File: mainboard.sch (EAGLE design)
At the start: 75 parts, among them Q3 MOSFET-PCHANNEL, Q4 MOSFET-PCHANNEL, T1 SINGLE_NCHAN_FET, T2 MOSFET_PCHAN_20A, T3 SINGLE_NCHAN_FET, T4 MOSFET_PCHAN_20A, T5 SINGLE_NCHAN_FET, T6 MOSFET_PCHAN_20A, U1 LT3688, U2 TEENSY_3.0+4, U3 RFM23BP, U4 HMC5883LSMD, U5 ITG-3200, U9 MIC803-31D3VM3TR

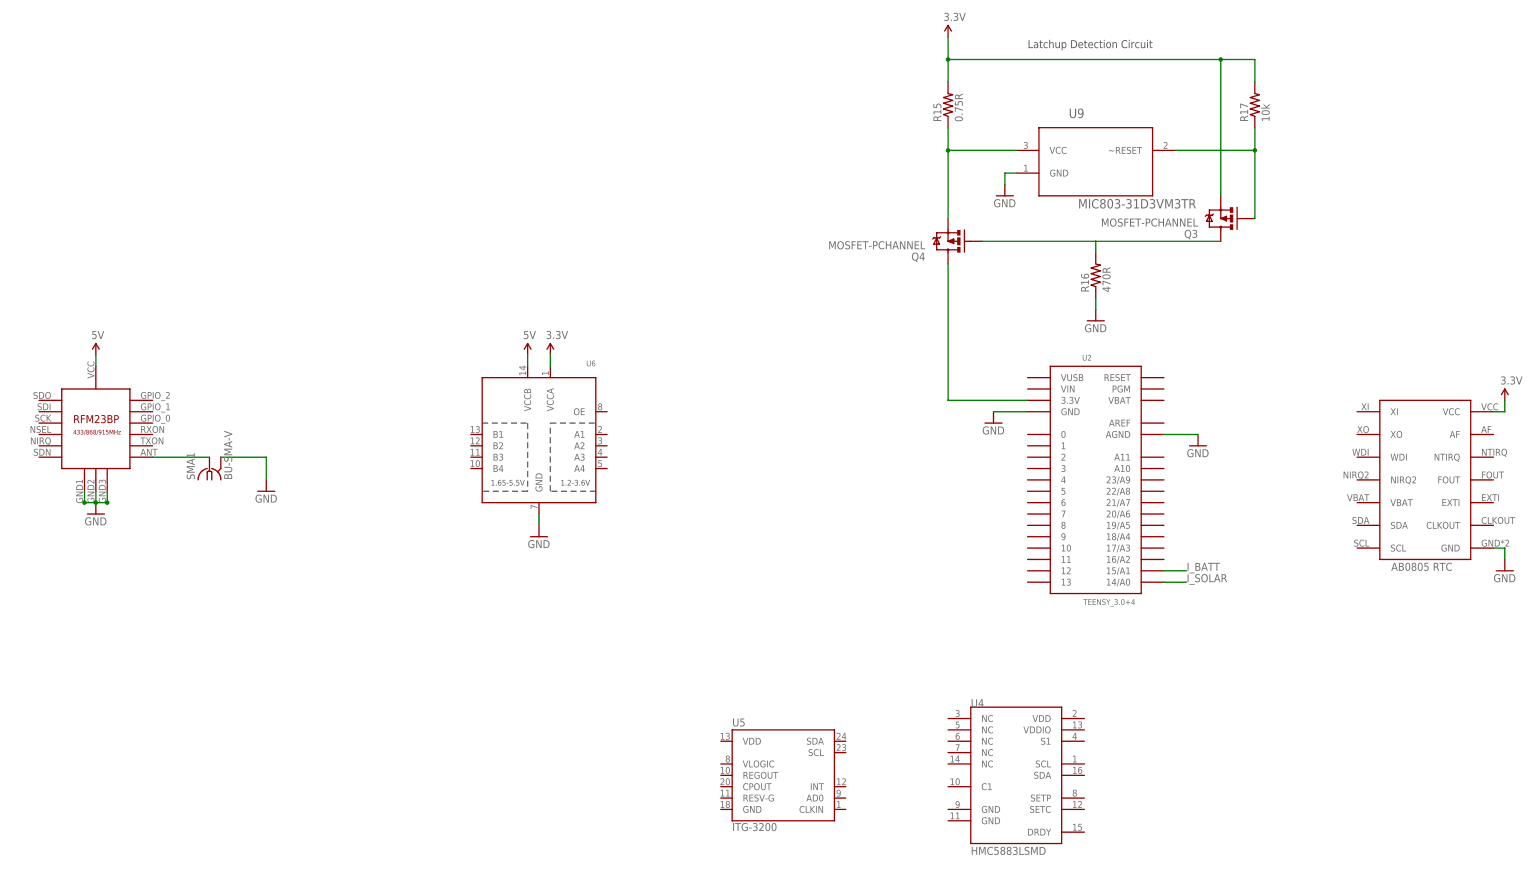
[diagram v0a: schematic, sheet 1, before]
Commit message: Mainboard layout work
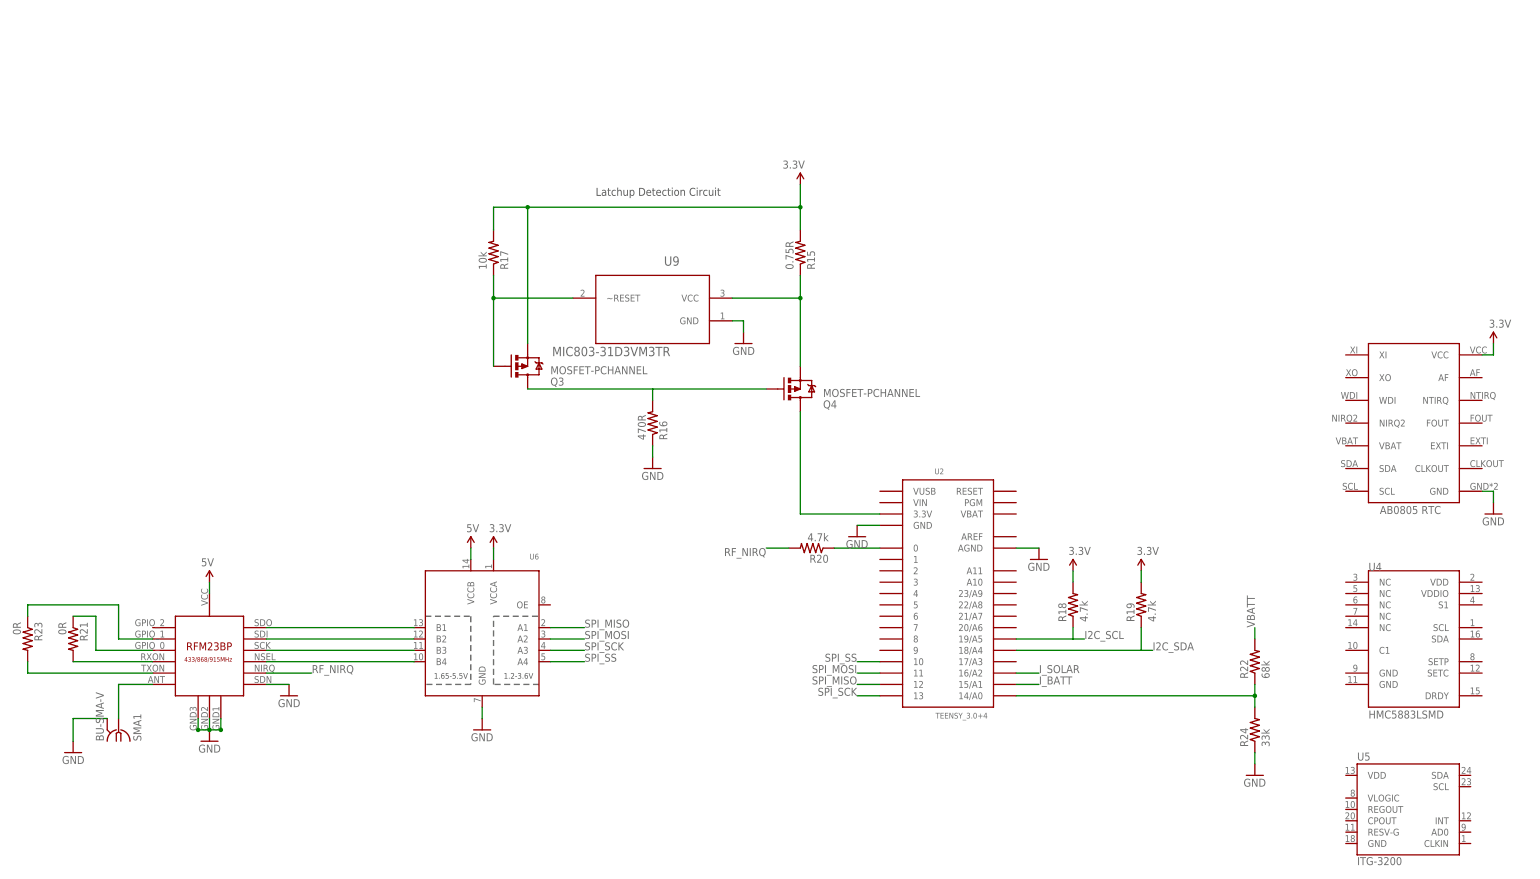
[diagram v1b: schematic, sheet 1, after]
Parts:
- added R18, R19, R20: 4.7k, SparkFun-Resistors:RESISTOR0805-RES
- added R21, R23: 0R, SparkFun-Resistors:RESISTOR0805-RES
- added R22: 68k, SparkFun-Resistors:RESISTOR0805-RES
- added R24: 33k, SparkFun-Resistors:RESISTOR0805-RES
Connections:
- new net I2C_SCL: R18.1, U2.19/A5
- new net I2C_SDA: R19.1, U2.18/A4
- new net N$28: U3.SDO, U6.B1
- new net N$29: U3.SDI, U6.B2
- new net N$30: U3.SCK, U6.B3
- new net N$31: U3.NSEL, U6.B4
- new net N$32: R20.1, U2.0
- new net N$33: R21.2, U3.RXON
- new net N$34: R21.1, U3.GPIO_0
- new net N$35: R23.2, U3.TXON
- new net N$36: R23.1, U3.GPIO_1
- new net N$37: R22.1, R24.2, U2.14/A0
- new net RF_NIRQ: R20.2, U3.NIRQ
- new net SPI_MISO: U2.12, U6.A1
- new net SPI_MOSI: U2.11, U6.A2
- new net SPI_SCK: U2.13, U6.A3
- new net SPI_SS: U2.10, U6.A4
- net 3.3V: now also R18.2, R19.2
- net GND: now also R24.1, U3.SDN
- net I_SOLAR: now also U2.16/A2; no longer U2.14/A0
- net VBATT: now also R22.2
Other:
- moved on the sheet: Q3, Q4, R15, R16, R17, SMA1, U2, U4, U5, U6, U9
